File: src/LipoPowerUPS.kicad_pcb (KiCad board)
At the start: 2 copper layers, 81 x 50 mm, 69 parts, among them J1 Battery, J2 Battery, J3 PowerSupply, J4 PowerSupply, J5 OUT, J6 OUT, Q1 HY4008, Q2 AO3401, Q3 AO3400, Q4 BCP56, SW1 BAT ON, SW2 BAT OFF, U2 LM324, U3 PC817, U5 MIC4428, U6 MB1S

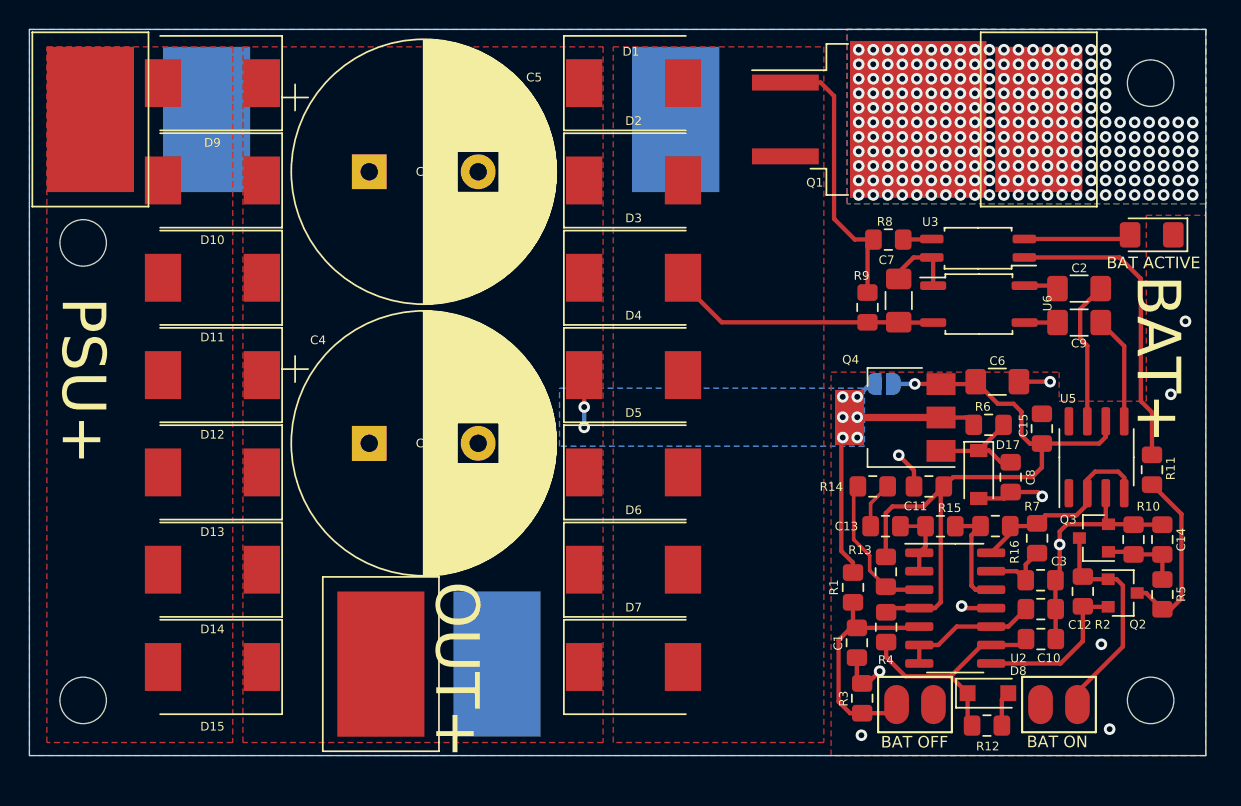
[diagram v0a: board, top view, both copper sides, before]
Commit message: Upload version V2.0
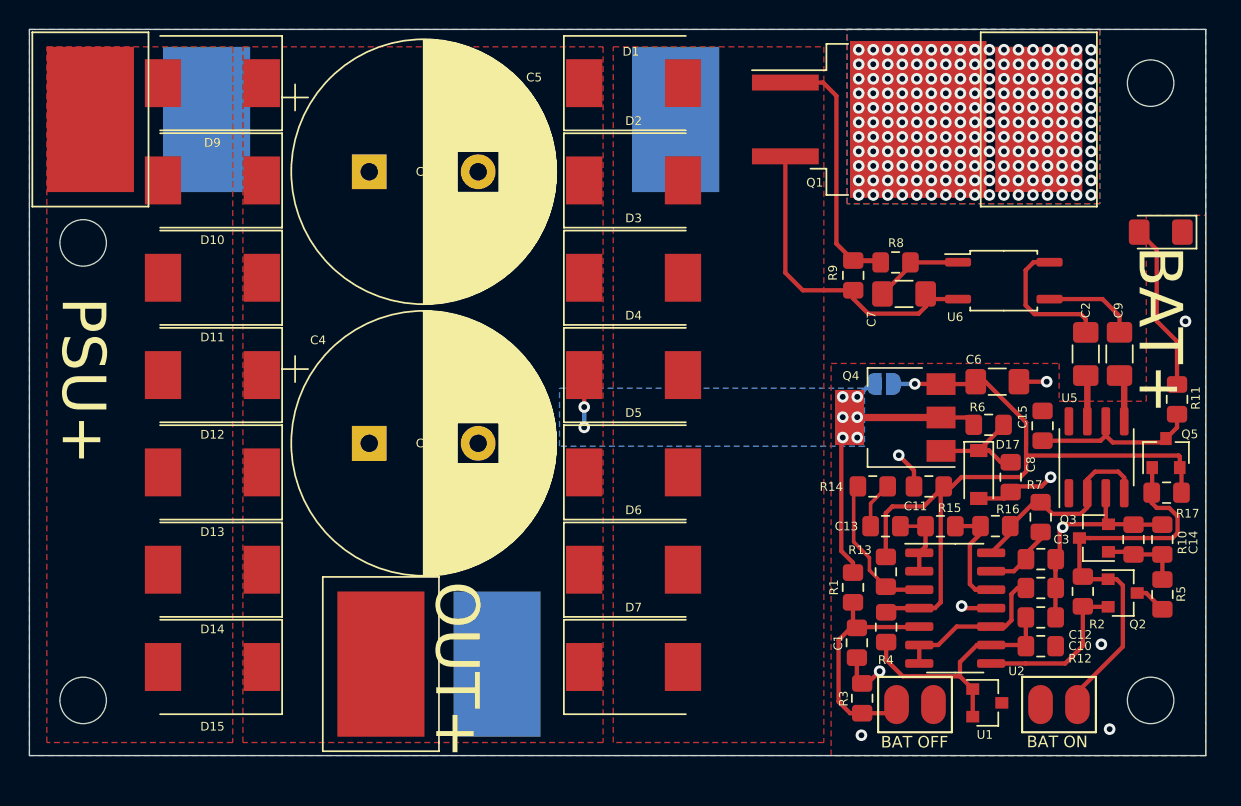
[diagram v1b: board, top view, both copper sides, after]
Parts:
- removed D16: BAT ACTIVE, LED_SMD:LED_1206_3216Metric_Pad1.42x1.75mm_HandSolder
- removed U3: PC817, Package_SO:SOP-4_4.4x2.6mm_P1.27mm
- added Q5: AO3401, Package_TO_SOT_SMD:SOT-23, F.Cu at (198.6, 92.5)
- added R17: 470K, Resistor_SMD:R_0805_2012Metric_Pad1.15x1.40mm_HandSolder, F.Cu at (198.6, 95.2)
- added U1: TL431DBZ, Package_TO_SOT_SMD:SOT-23, F.Cu at (186.3, 109.7)
- C10: value 100n -> 1u
- D8: value 3V3 -> BAT ACTIVE; footprint Diode_SMD:D_SOD-123F -> LED_SMD:LED_1206_3216Metric_Pad1.42x1.75mm_HandSolder
- R1: value 47K -> 120K/51K
- R12: value 680K -> 820K
- R13, R14: value 33K -> 100K
- R3: value 10K -> 18K
- R4: value 6K8 -> 3K3
- R9: value 470K -> 330K
- moved D8 33.9 mm to (198.2, 77.3), turned to 180 degrees
- moved R12 6.60 mm to (189.9, 105.8)
- moved R11 5.15 mm to (199.3, 88.8)
- moved C2 4.53 mm to (193.0, 85.6), turned to 270 degrees
- moved C9 3.52 mm to (195.4, 85.6), turned to 270 degrees
- moved R9 2.41 mm to (177.0, 80.2)
- moved U6 2.35 mm to (187.4, 80.6)
- moved R8 1.65 mm to (179.9, 79.3)
- moved C10 1.49 mm to (189.9, 103.8)
- moved R7 1.47 mm to (189.9, 96.9)
- moved C3 1.45 mm to (189.9, 99.8)
- moved C12 1.45 mm to (189.9, 101.8)
- moved C7 0.58 mm to (180.5, 81.5), turned to 0 degrees
- moved C15 0.20 mm to (190.1, 90.6)
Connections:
- C10 pad 1: /3V3_REF -> /2V5_REF
- C15 pad 2: +12V -> /GATE_VCC
- D8 pad 1: /3V3_REF -> GND
- D8 pad 2: GND -> Net-(D8-Pad2)
- R11 pad 1: Net-(Q2-Pad3) -> /GATE_VCC
- R11 pad 2: /EN_BAT -> Net-(D8-Pad2)
- R12 pad 2: /3V3_REF -> /2V5_REF
- R4 pad 1: /3V3_REF -> /2V5_REF
- R8 pad 2: Net-(R8-Pad2) -> Net-(C7-Pad1)
- U2 pad 9: /3V3_REF -> /2V5_REF
- U5 pad 6: +12V -> /GATE_VCC
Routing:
- net /EN_BAT: track 21.1 -> 0.00 mm
- net /2V5_REF: track 0.00 -> 17.9 mm
- net /3V3_REF: track 16.3 -> 0.00 mm
- net Net-(Q2-Pad1): track 15.0 -> 27.7 mm
- net /GATE_VCC: track 0.00 -> 11.9 mm
- net Net-(D8-Pad2): track 0.00 -> 11.6 mm
- net Net-(Q2-Pad3): track 12.5 -> 2.20 mm
- net Net-(D16-Pad2): track 7.40 -> 0.00 mm
- net Net-(C2-Pad1): track 2.34 -> 9.73 mm
- net /CP1: track 9.93 -> 3.19 mm
- net +12V: track 47.5 -> 52.9 mm
- net /CP2: track 7.47 -> 3.29 mm
- net Net-(C9-Pad1): track 2.26 -> 6.42 mm
- net /MOSFET_S: track 18.7 -> 22.6 mm
- net GND: track 37.7 -> 33.9 mm, vias 11 -> 10
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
